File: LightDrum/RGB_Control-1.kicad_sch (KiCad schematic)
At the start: 25 parts, among them Q10 PMXB43UNEZ, Q11 PMXB43UNEZ, Q4 PMXB43UNEZ, Q5 PMXB43UNEZ, Q6 PMXB43UNEZ, Q7 PMXB43UNEZ, Q8 PMXB43UNEZ, Q9 PMXB43UNEZ, U9 PCA9634_TSSOP20

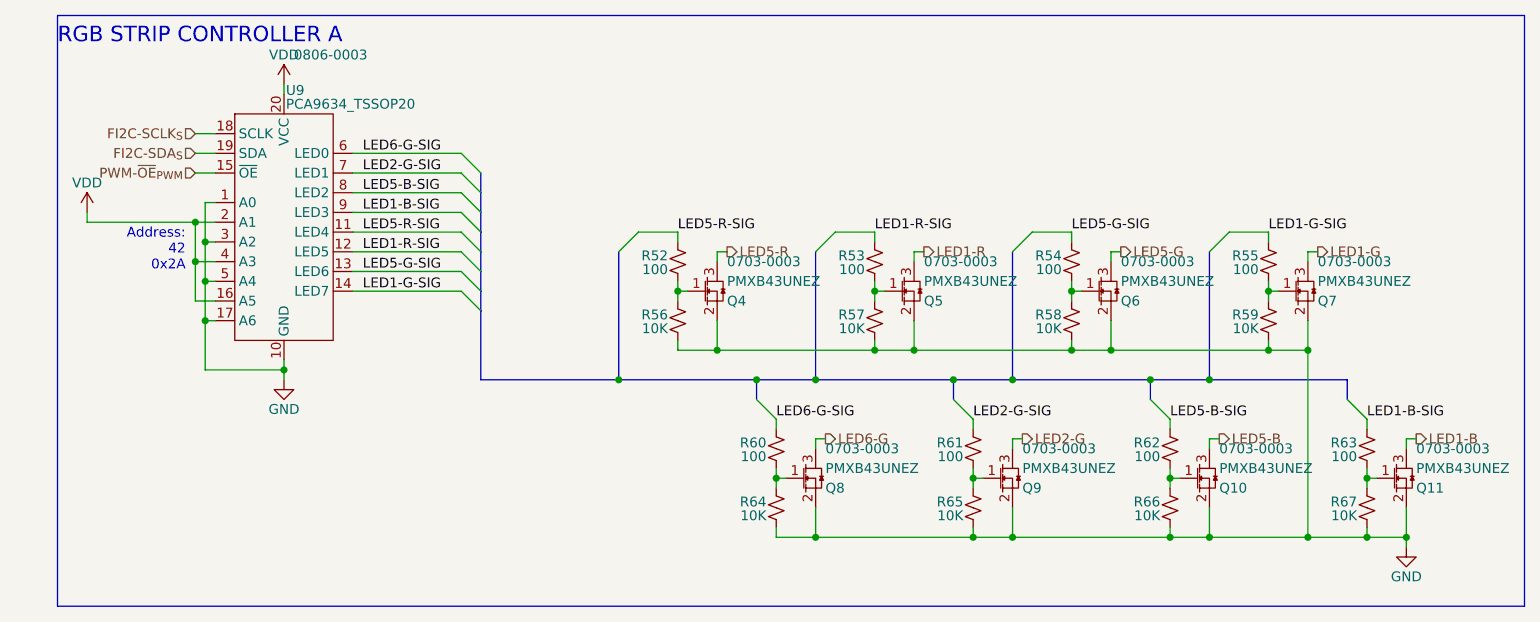
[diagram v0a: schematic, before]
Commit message: Minor fixes and cleanup - REV11
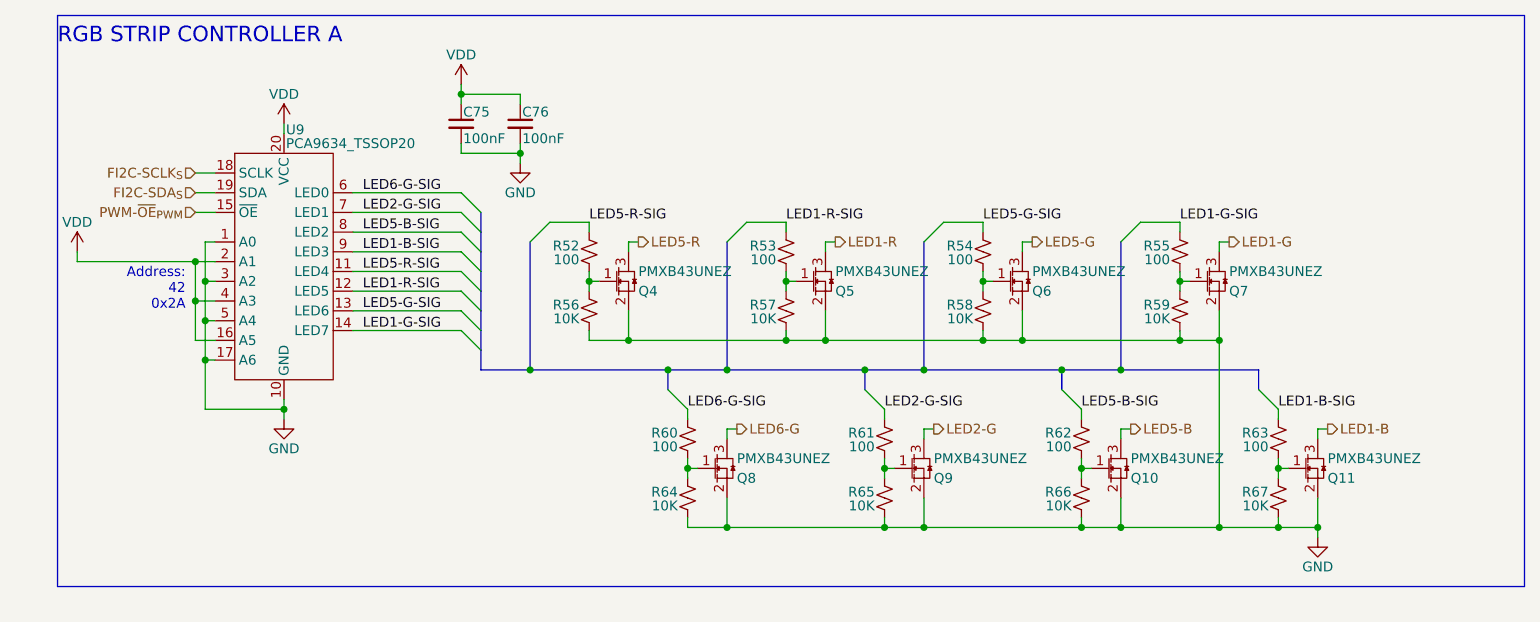
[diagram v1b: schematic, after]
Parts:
- added C75, C76: 100nF, Capacitor_SMD:C_0402_1005Metric, symbol Daxxn_Device:C
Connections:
- net GND: now also C75.2, C76.2
- net VDD: now also C75.1, C76.1
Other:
- moved on the sheet: Q10, Q11, Q4, Q5, Q6, Q7, Q8, Q9, R52, R53, R54, R55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
